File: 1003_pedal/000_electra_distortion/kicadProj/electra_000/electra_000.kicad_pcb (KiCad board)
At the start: 2 copper layers, 17 parts, among them J1 AudioJack2, J2 AudioJack2, Q1 Q_NPN_BCE, SW1 SW_Slide_DPDT

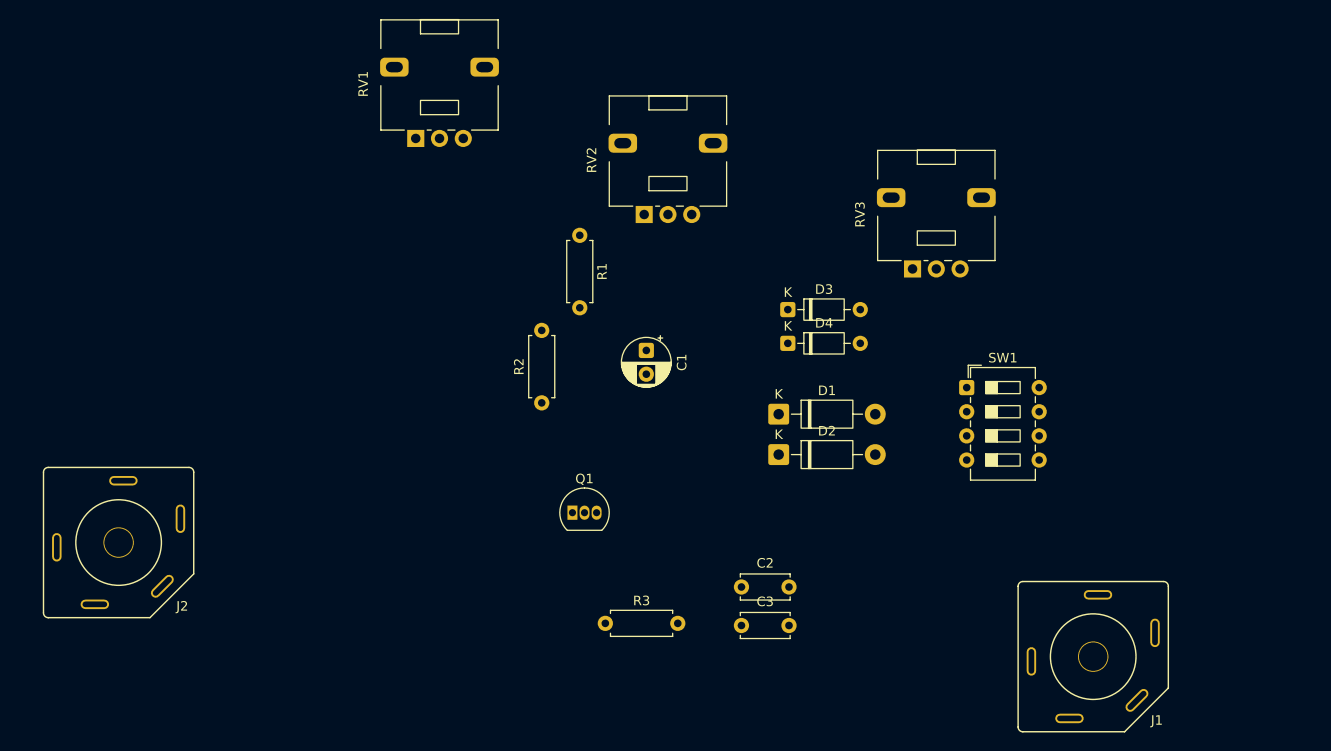
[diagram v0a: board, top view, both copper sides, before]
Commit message: library added
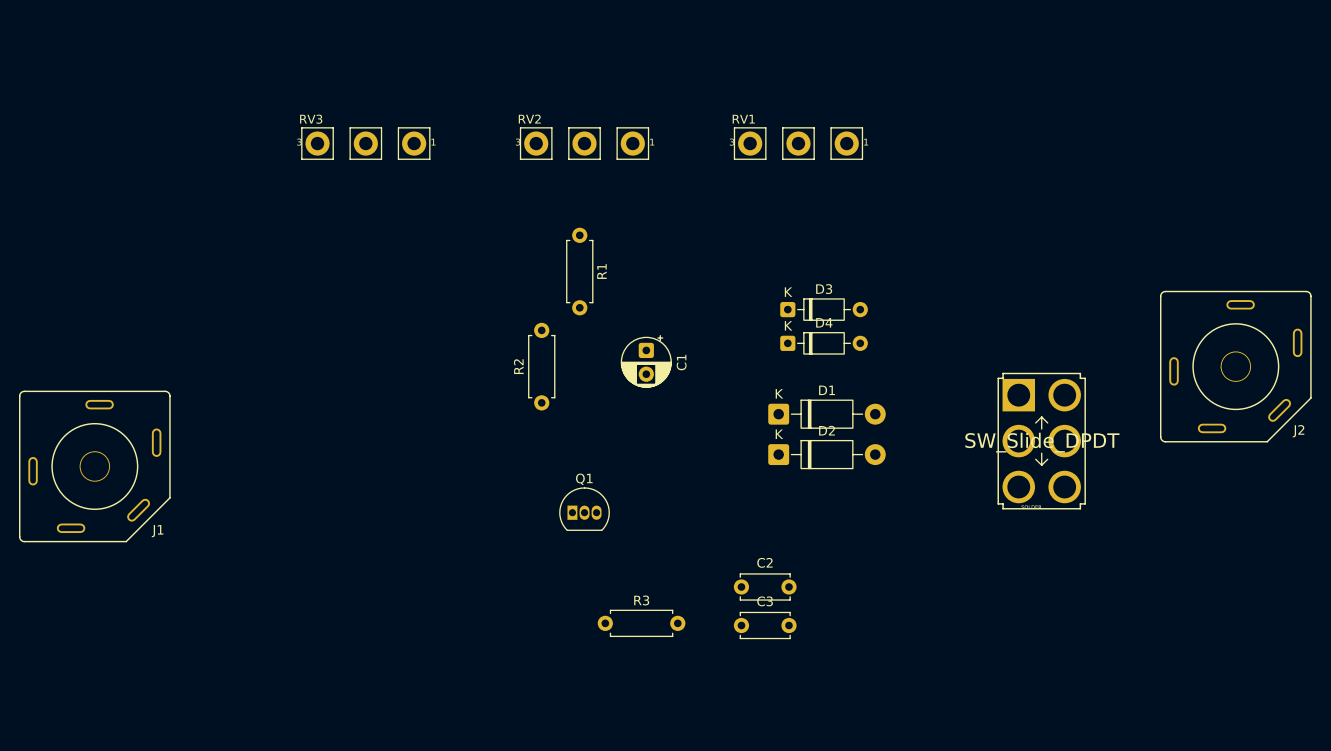
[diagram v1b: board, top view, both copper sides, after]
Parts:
- RV1, RV2, RV3: footprint Potentiometer_THT:Potentiometer_Alps_RK09L_Single_Vertical -> Monkey_Riot_Pedals_Library:POT_16MM
- SW1: footprint Button_Switch_THT:SW_DIP_SPSTx04_Slide_6.7x11.72mm_W7.62mm_P2.54mm_LowProfile -> Monkey_Riot_Pedals_Library:DPDT.LUGS
- moved J2 118.9 mm to (164.0, 80.0)
- moved J1 106.9 mm to (44.0, 90.5)
- moved RV3 59.0 mm to (72.5, 56.5), turned to 0 degrees
- moved RV1 40.3 mm to (118.0, 56.5), turned to 0 degrees
- moved RV2 9.75 mm to (95.5, 56.5), turned to 0 degrees
- moved SW1 9.69 mm to (143.6, 87.8)
